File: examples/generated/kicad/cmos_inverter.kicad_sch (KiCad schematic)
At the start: 4 parts

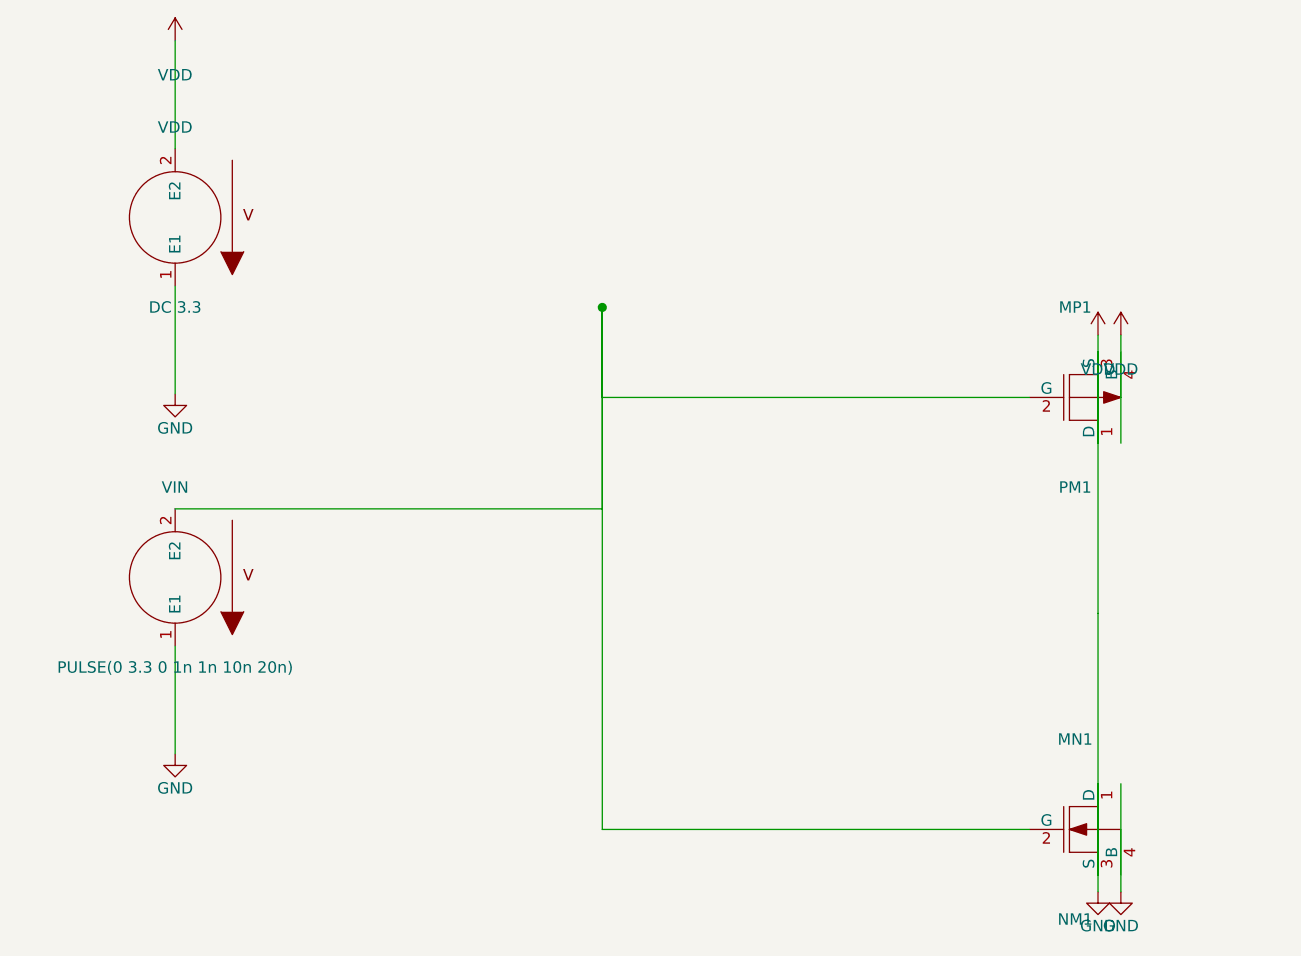
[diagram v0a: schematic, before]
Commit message: Attempt to correct strange wiring.
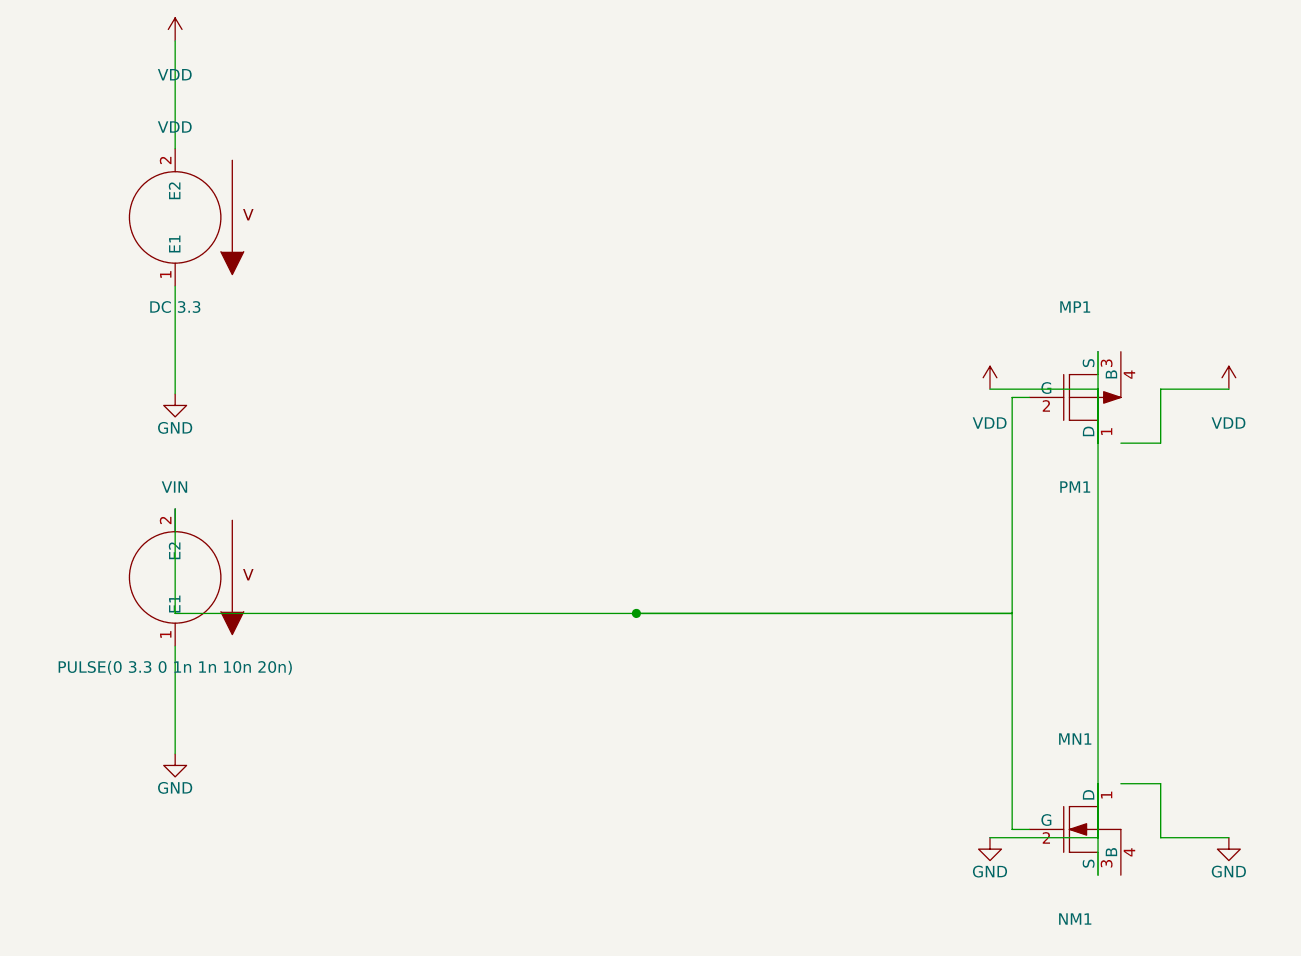
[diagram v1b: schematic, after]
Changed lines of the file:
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@@
     )
   )
-  (symbol (lib_id "VCC") (at 152.54 83.08 0) (unit 1)
+  (symbol (lib_id "VCC") (at 140.54 89.08 0) (unit 1)
     (in_bom yes) (on_board yes)
-    (property "Reference" "#PWR0004" (at 152.54 79.27 0)
+    (property "Reference" "#PWR0004" (at 140.54 85.27 0)
       (effects (font (size 1.27 1.27)) hide)
     )
-    (property "Value" "VDD" (at 152.54 86.89 0)
+    (property "Value" "VDD" (at 140.54 92.89 0)
       (effects (font (size 1.27 1.27)))
     )
@@
     )
   )
-  (symbol (lib_id "VCC") (at 155.08 83.08 0) (unit 1)
+  (symbol (lib_id "VCC") (at 167.08 89.08 0) (unit 1)
     (in_bom yes) (on_board yes)
-    (property "Reference" "#PWR0005" (at 155.08 79.27 0)
+    (property "Reference" "#PWR0005" (at 167.08 85.27 0)
       (effects (font (size 1.27 1.27)) hide)
     )
-    (property "Value" "VDD" (at 155.08 86.89 0)
+    (property "Value" "VDD" (at 167.08 92.89 0)
       (effects (font (size 1.27 1.27)))
     )
@@
     )
   )
-  (symbol (lib_id "GND") (at 152.54 144.92 0) (unit 1)
+  (symbol (lib_id "GND") (at 140.54 138.92 0) (unit 1)
     (in_bom yes) (on_board yes)
-    (property "Reference" "#PWR0006" (at 152.54 141.10999999999999 0)
+    (property "Reference" "#PWR0006" (at 140.54 135.10999999999999 0)
       (effects (font (size 1.27 1.27)) hide)
     )
-    (property "Value" "GND" (at 152.54 148.73 0)
+    (property "Value" "GND" (at 140.54 142.73 0)
       (effects (font (size 1.27 1.27)))
     )
@@
     )
   )
-  (symbol (lib_id "GND") (at 155.08 144.92 0) (unit 1)
+  (symbol (lib_id "GND") (at 167.08 138.92 0) (unit 1)
     (in_bom yes) (on_board yes)
-    (property "Reference" "#PWR0007" (at 155.08 141.10999999999999 0)
+    (property "Reference" "#PWR0007" (at 167.08 135.10999999999999 0)
       (effects (font (size 1.27 1.27)) hide)
     )
-    (property "Value" "GND" (at 155.08 148.73 0)
+    (property "Value" "GND" (at 167.08 142.73 0)
       (effects (font (size 1.27 1.27)))
     )
@@
     (stroke (width 0) (type solid) (color 0 0 0 0))
   )
-  (wire (pts (xy 152.54 95.08) (xy 152.54 83.08))
+  (wire (pts (xy 152.54 95.08) (xy 152.54 89.08))
     (stroke (width 0) (type solid) (color 0 0 0 0))
   )
-  (wire (pts (xy 155.08 95.08) (xy 155.08 83.08))
+  (wire (pts (xy 152.54 89.08) (xy 140.54 89.08))
     (stroke (width 0) (type solid) (color 0 0 0 0))
   )
-  (wire (pts (xy 152.54 132.92) (xy 152.54 144.92))
+  (wire (pts (xy 155.08 95.08) (xy 159.50 95.08))
     (stroke (width 0) (type solid) (color 0 0 0 0))
   )
-  (wire (pts (xy 155.08 132.92) (xy 155.08 144.92))
+  (wire (pts (xy 159.50 95.08) (xy 159.50 89.08))
     (stroke (width 0) (type solid) (color 0 0 0 0))
   )
-  (wire (pts (xy 50.00 102.38) (xy 97.46 102.38))
+  (wire (pts (xy 159.50 89.08) (xy 167.08 89.08))
     (stroke (width 0) (type solid) (color 0 0 0 0))
   )
-  (wire (pts (xy 97.46 102.38) (xy 97.46 80.00))
+  (wire (pts (xy 152.54 132.92) (xy 152.54 138.92))
     (stroke (width 0) (type solid) (color 0 0 0 0))
   )
-  (wire (pts (xy 144.92 90.00) (xy 97.46 90.00))
+  (wire (pts (xy 152.54 138.92) (xy 140.54 138.92))
     (stroke (width 0) (type solid) (color 0 0 0 0))
   )
-  (wire (pts (xy 97.46 90.00) (xy 97.46 80.00))
+  (wire (pts (xy 155.08 132.92) (xy 159.50 132.92))
     (stroke (width 0) (type solid) (color 0 0 0 0))
   )
-  (wire (pts (xy 144.92 138.00) (xy 97.46 138.00))
+  (wire (pts (xy 159.50 132.92) (xy 159.50 138.92))
     (stroke (width 0) (type solid) (color 0 0 0 0))
   )
-  (wire (pts (xy 97.46 138.00) (xy 97.46 80.00))
+  (wire (pts (xy 159.50 138.92) (xy 167.08 138.92))
     (stroke (width 0) (type solid) (color 0 0 0 0))
   )
-  (wire (pts (xy 152.54 84.92) (xy 152.54 114.00))
+  (wire (pts (xy 50.00 102.38) (xy 50.00 114.00))
     (stroke (width 0) (type solid) (color 0 0 0 0))
   )
-  (wire (pts (xy 152.54 143.08) (xy 152.54 114.00))
+  (wire (pts (xy 50.00 114.00) (xy 101.25 114.00))
     (stroke (width 0) (type solid) (color 0 0 0 0))
   )
-  (junction (at 97.46 80.00) (diameter 1.016) (color 0 0 0 0))
+  (wire (pts (xy 144.92 90.00) (xy 143.00 90.00))
+    (stroke (width 0) (type solid) (color 0 0 0 0))
+  )
+  (wire (pts (xy 143.00 90.00) (xy 143.00 114.00))
+    (stroke (width 0) (type solid) (color 0 0 0 0))
+  )
+  (wire (pts (xy 143.00 114.00) (xy 101.25 114.00))
+    (stroke (width 0) (type solid) (color 0 0 0 0))
+  )
+  (wire (pts (xy 144.92 138.00) (xy 143.00 138.00))
+    (stroke (width 0) (type solid) (color 0 0 0 0))
+  )
+  (wire (pts (xy 143.00 138.00) (xy 143.00 114.00))
+    (stroke (width 0) (type solid) (color 0 0 0 0))
+  )
+  (wire (pts (xy 143.00 114.00) (xy 101.25 114.00))
+    (stroke (width 0) (type solid) (color 0 0 0 0))
+  )
+  (wire (pts (xy 152.54 84.92) (xy 152.54 143.08))
+    (stroke (width 0) (type solid) (color 0 0 0 0))
+  )
+  (junction (at 101.25 114.00) (diameter 1.016) (color 0 0 0 0))
   (sheet_instances
     (path "/" (page "1"))

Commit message: Attempt shape and wiring fixes again.
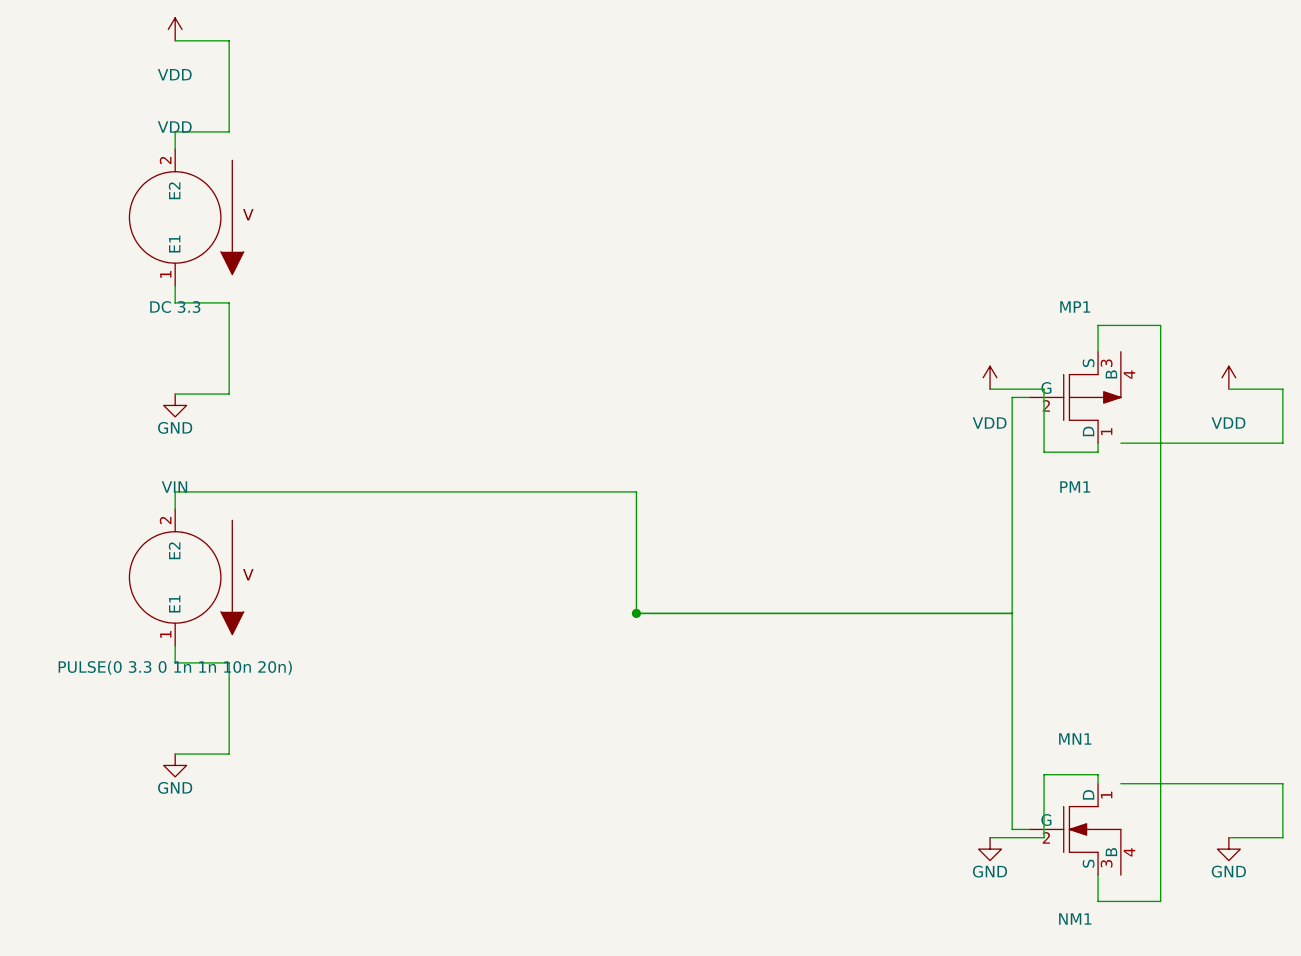
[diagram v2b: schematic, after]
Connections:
- net GND: no longer MN1.3 (S), MP1.1 (D), MP1.3 (S), VDD.2 (E2)
- new net: MN1.3 (S), MP1.3 (S)
- new net VDD: MP1.1 (D), VDD.2 (E2)
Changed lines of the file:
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@@
     )
   )
-  (wire (pts (xy 50.00 62.38) (xy 50.00 50.38))
+  (wire (pts (xy 50.00 62.38) (xy 50.00 60.50))
     (stroke (width 0) (type solid) (color 0 0 0 0))
   )
-  (wire (pts (xy 50.00 77.62) (xy 50.00 89.62))
+  (wire (pts (xy 50.00 60.50) (xy 56.00 60.50))
     (stroke (width 0) (type solid) (color 0 0 0 0))
   )
-  (wire (pts (xy 50.00 117.62) (xy 50.00 129.62))
+  (wire (pts (xy 56.00 60.50) (xy 56.00 50.38))
     (stroke (width 0) (type solid) (color 0 0 0 0))
   )
-  (wire (pts (xy 152.54 95.08) (xy 152.54 89.08))
+  (wire (pts (xy 56.00 50.38) (xy 50.00 50.38))
     (stroke (width 0) (type solid) (color 0 0 0 0))
   )
-  (wire (pts (xy 152.54 89.08) (xy 140.54 89.08))
+  (wire (pts (xy 50.00 77.62) (xy 50.00 79.50))
     (stroke (width 0) (type solid) (color 0 0 0 0))
   )
-  (wire (pts (xy 155.08 95.08) (xy 159.50 95.08))
+  (wire (pts (xy 50.00 79.50) (xy 56.00 79.50))
     (stroke (width 0) (type solid) (color 0 0 0 0))
   )
-  (wire (pts (xy 159.50 95.08) (xy 159.50 89.08))
+  (wire (pts (xy 56.00 79.50) (xy 56.00 89.62))
     (stroke (width 0) (type solid) (color 0 0 0 0))
   )
-  (wire (pts (xy 159.50 89.08) (xy 167.08 89.08))
+  (wire (pts (xy 56.00 89.62) (xy 50.00 89.62))
     (stroke (width 0) (type solid) (color 0 0 0 0))
   )
-  (wire (pts (xy 152.54 132.92) (xy 152.54 138.92))
+  (wire (pts (xy 50.00 117.62) (xy 50.00 119.50))
     (stroke (width 0) (type solid) (color 0 0 0 0))
   )
-  (wire (pts (xy 152.54 138.92) (xy 140.54 138.92))
+  (wire (pts (xy 50.00 119.50) (xy 56.00 119.50))
     (stroke (width 0) (type solid) (color 0 0 0 0))
   )
-  (wire (pts (xy 155.08 132.92) (xy 159.50 132.92))
+  (wire (pts (xy 56.00 119.50) (xy 56.00 129.62))
     (stroke (width 0) (type solid) (color 0 0 0 0))
   )
-  (wire (pts (xy 159.50 132.92) (xy 159.50 138.92))
+  (wire (pts (xy 56.00 129.62) (xy 50.00 129.62))
     (stroke (width 0) (type solid) (color 0 0 0 0))
   )
-  (wire (pts (xy 159.50 138.92) (xy 167.08 138.92))
+  (wire (pts (xy 152.54 95.08) (xy 152.54 96.08))
     (stroke (width 0) (type solid) (color 0 0 0 0))
   )
-  (wire (pts (xy 50.00 102.38) (xy 50.00 114.00))
+  (wire (pts (xy 152.54 96.08) (xy 146.54 96.08))
     (stroke (width 0) (type solid) (color 0 0 0 0))
   )
-  (wire (pts (xy 50.00 114.00) (xy 101.25 114.00))
+  (wire (pts (xy 146.54 96.08) (xy 146.54 89.08))
+    (stroke (width 0) (type solid) (color 0 0 0 0))
+  )
+  (wire (pts (xy 146.54 89.08) (xy 140.54 89.08))
+    (stroke (width 0) (type solid) (color 0 0 0 0))
+  )
+  (wire (pts (xy 155.08 95.08) (xy 173.08 95.08))
+    (stroke (width 0) (type solid) (color 0 0 0 0))
+  )
+  (wire (pts (xy 173.08 95.08) (xy 173.08 89.08))
+    (stroke (width 0) (type solid) (color 0 0 0 0))
+  )
+  (wire (pts (xy 173.08 89.08) (xy 167.08 89.08))
+    (stroke (width 0) (type solid) (color 0 0 0 0))
+  )
+  (wire (pts (xy 152.54 132.92) (xy 152.54 131.92))
+    (stroke (width 0) (type solid) (color 0 0 0 0))
+  )
+  (wire (pts (xy 152.54 131.92) (xy 146.54 131.92))
+    (stroke (width 0) (type solid) (color 0 0 0 0))
+  )
+  (wire (pts (xy 146.54 131.92) (xy 146.54 138.92))
+    (stroke (width 0) (type solid) (color 0 0 0 0))
+  )
+  (wire (pts (xy 146.54 138.92) (xy 140.54 138.92))
+    (stroke (width 0) (type solid) (color 0 0 0 0))
+  )
+  (wire (pts (xy 155.08 132.92) (xy 173.08 132.92))
+    (stroke (width 0) (type solid) (color 0 0 0 0))
+  )
+  (wire (pts (xy 173.08 132.92) (xy 173.08 138.92))
+    (stroke (width 0) (type solid) (color 0 0 0 0))
+  )
+  (wire (pts (xy 173.08 138.92) (xy 167.08 138.92))
+    (stroke (width 0) (type solid) (color 0 0 0 0))
+  )
+  (wire (pts (xy 50.00 102.38) (xy 50.00 100.50))
+    (stroke (width 0) (type solid) (color 0 0 0 0))
+  )
+  (wire (pts (xy 50.00 100.50) (xy 101.25 100.50))
+    (stroke (width 0) (type solid) (color 0 0 0 0))
+  )
+  (wire (pts (xy 101.25 100.50) (xy 101.25 114.00))
     (stroke (width 0) (type solid) (color 0 0 0 0))
   )
@@
     (stroke (width 0) (type solid) (color 0 0 0 0))
   )
-  (wire (pts (xy 152.54 84.92) (xy 152.54 143.08))
+  (wire (pts (xy 152.54 84.92) (xy 152.54 82.00))
     (stroke (width 0) (type solid) (color 0 0 0 0))
   )
+  (wire (pts (xy 152.54 82.00) (xy 159.50 82.00))
+    (stroke (width 0) (type solid) (color 0 0 0 0))
+  )
+  (wire (pts (xy 159.50 82.00) (xy 159.50 146.00))
+    (stroke (width 0) (type solid) (color 0 0 0 0))
+  )
+  (wire (pts (xy 159.50 146.00) (xy 152.54 146.00))
+    (stroke (width 0) (type solid) (color 0 0 0 0))
+  )
+  (wire (pts (xy 152.54 146.00) (xy 152.54 143.08))
+    (stroke (width 0) (type solid) (color 0 0 0 0))
+  )
